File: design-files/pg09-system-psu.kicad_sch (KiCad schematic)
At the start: 9 parts, among them J1 ATX-24, J802 #PS_ON, J803 PSU-CTRL console, SW201 Power, U801 Adafruit_Metro_Mini

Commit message: Add Mouser part # for ATX PSU connector.
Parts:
- J1: Mouser (none) -> 538-39-28-1243
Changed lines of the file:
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@@
+      (effects (font (size 1.27 1.27)) hide)
+    )
+    (property "Mouser" "538-39-28-1243" (at 142.24 51.435 0)
+      (effects (font (size 1.27 1.27)) hide)
+    )
+    (property "Field5" "" (at 142.24 51.435 0)
       (effects (font (size 1.27 1.27)) hide)
     )

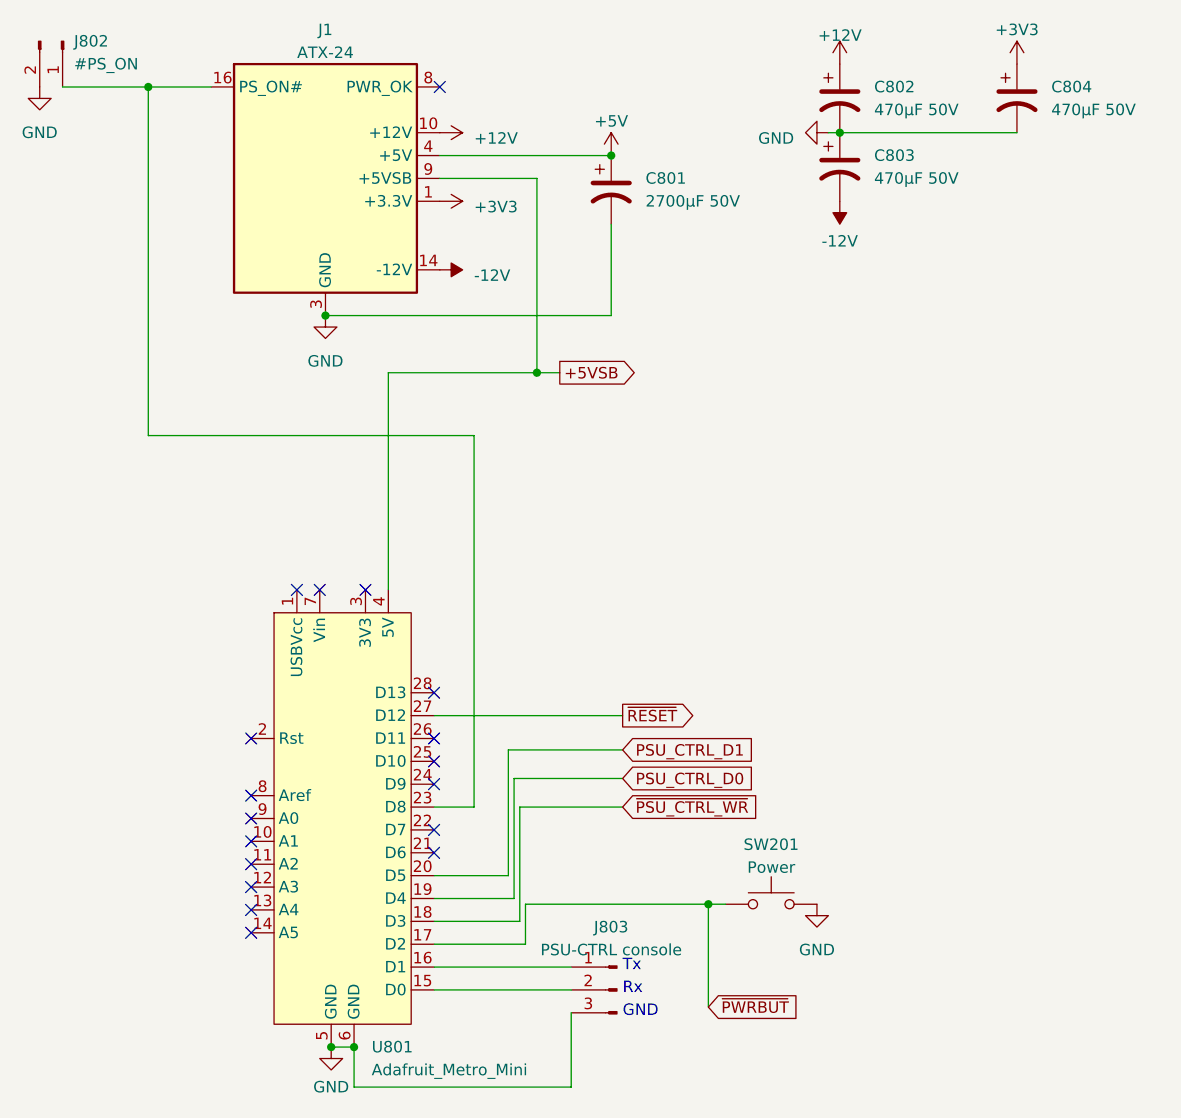
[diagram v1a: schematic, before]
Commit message: Add Power LED.  Tweak UART interface connectors.
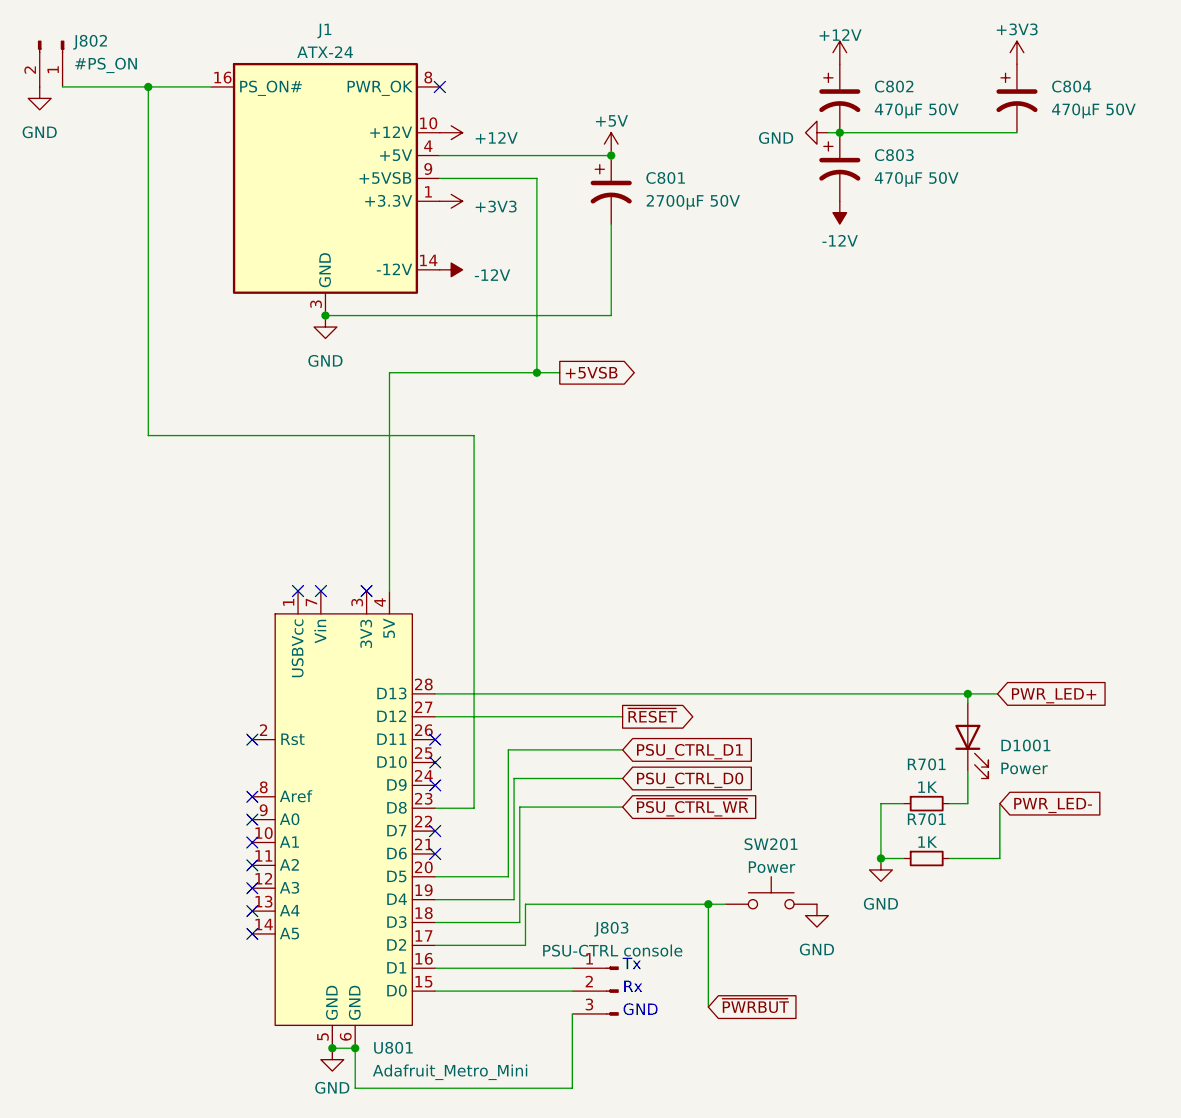
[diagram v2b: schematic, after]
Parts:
- added D1001: Power, LED_THT:LED_D3.0mm, symbol Device:LED
- added R701 (x2): 1K, Resistor_THT:R_Axial_DIN0207_L6.3mm_D2.5mm_P7.62mm_Horizontal, symbol Device:R_Small
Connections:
- net GND: now also R701.1, R701.1
- net PWR_LED+: now reaches U801.28 (D13)
- net PWR_LED+: now also D1001.2 (A)
- new net: D1001.1 (K), R701.2
- new net PWR_LED-: R701.2
- no-connect marks 18 -> 17
